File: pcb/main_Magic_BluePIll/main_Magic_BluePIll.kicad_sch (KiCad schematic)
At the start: 46 parts, among them J1 PW, J2 MPU6050, J3 ST_Link, J4 LiPo, J5 ESC, J9 Sensors, Q1 IRLML2502, SW1 Power_SW, SW4 BUTTON_Push, U1 BluePill_SWD_Breakout, U2 AMS1117CD-3.3, U6 CN3905

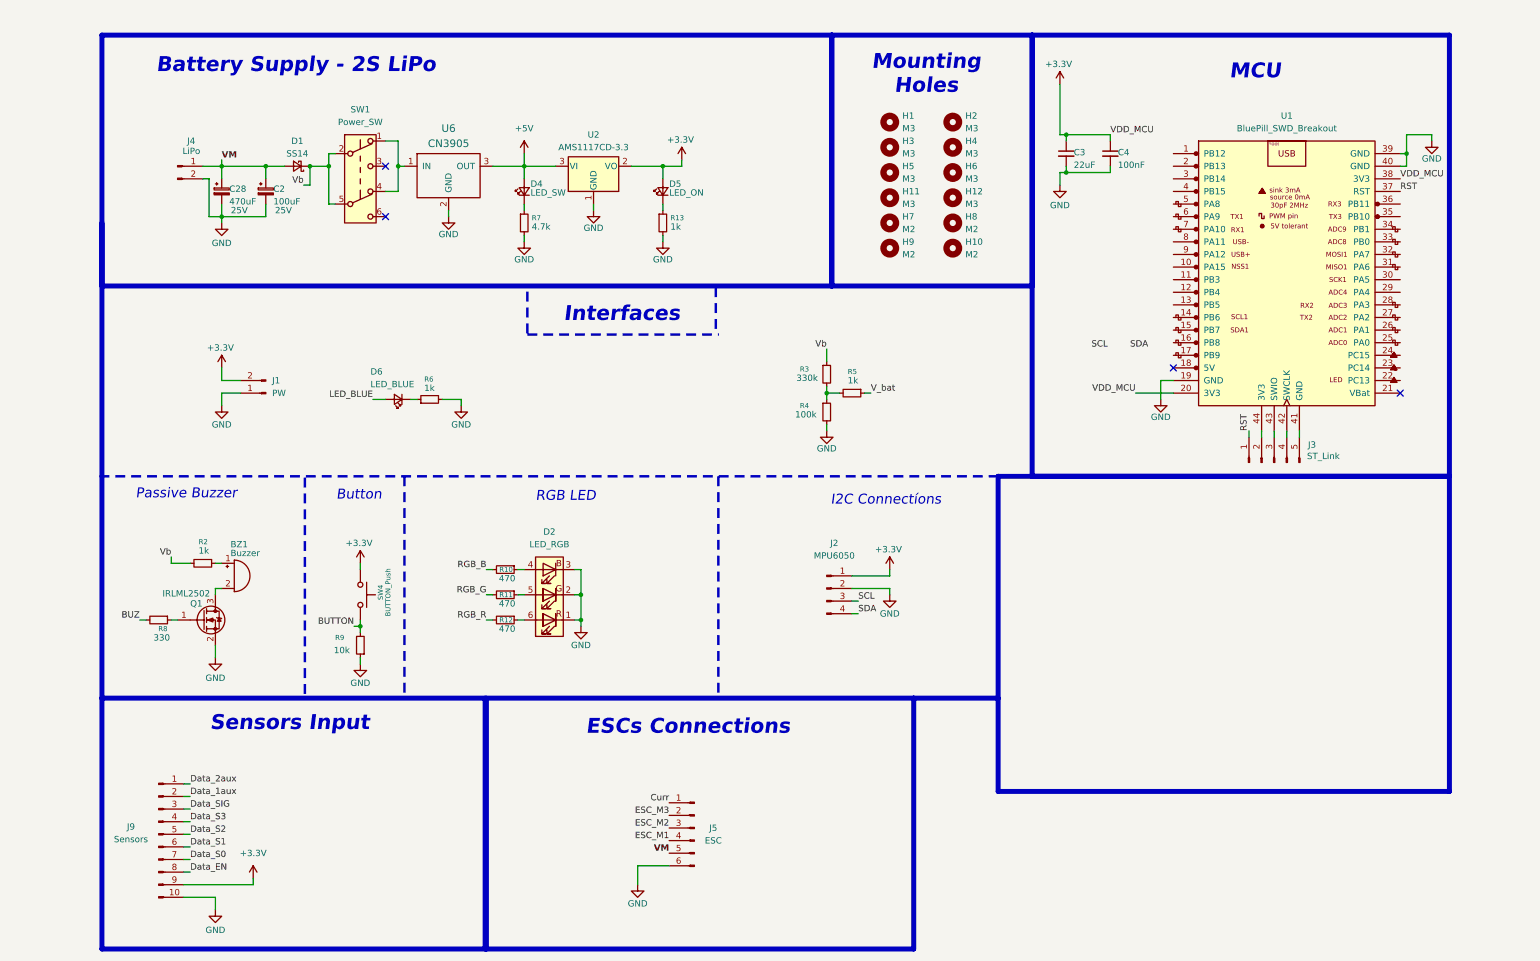
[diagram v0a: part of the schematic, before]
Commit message: bluepill pcb
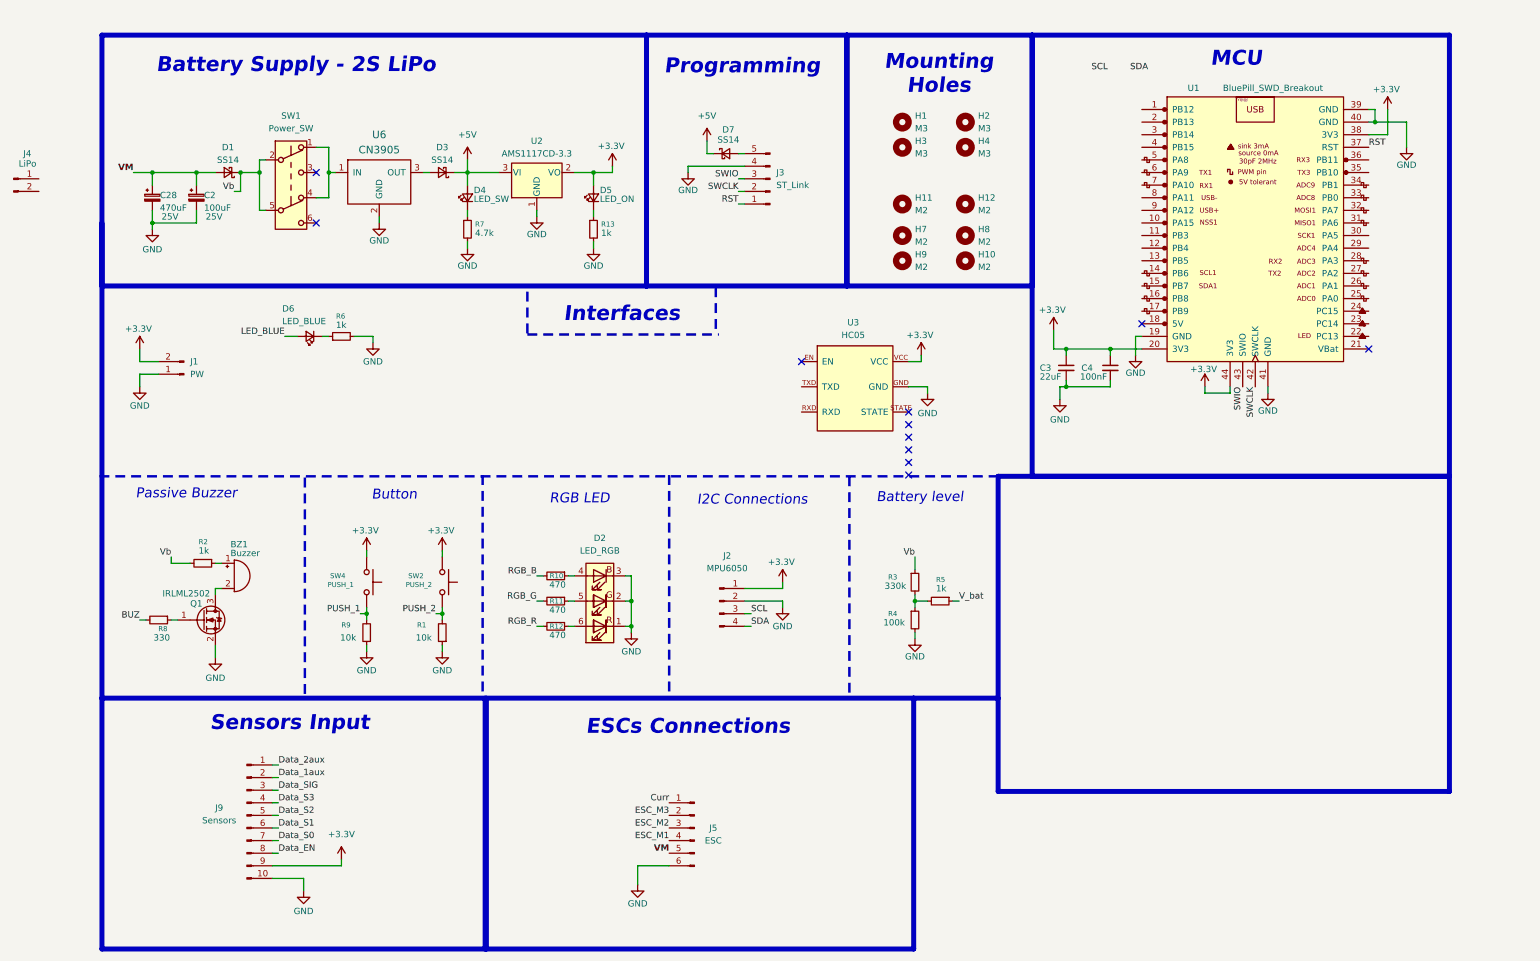
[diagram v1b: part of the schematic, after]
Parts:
- removed H5, H6: M3, MountingHole:MountingHole_3mm, symbol Mechanical:MountingHole
- added D3, D7: SS14, Diode_SMD:D_SMA, symbol Device:D_Schottky_Small
- added R1: 10k, Resistor_SMD:R_0805_2012Metric, symbol Device:R_Small
- added SW2: PUSH_2, MixLib:SW_Push_Sw-3424p_Handsolder, symbol Switch:SW_Push
- added U3: HC05, MixLib:HC05, symbol MixLib:HC05
- H11, H12: value M3 -> M2; footprint MountingHole:MountingHole_3mm -> MountingHole:MountingHole_2.2mm_M2
- J3: footprint Connector_PinHeader_2.54mm:PinHeader_1x05_P2.54mm_Horizontal -> Connector_PinHeader_2.54mm:PinHeader_1x05_P2.54mm_Vertical
- SW4: value BUTTON_Push -> PUSH_1
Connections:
- net +3.3V: now also U1.44 (3V3), SW2.1, U3.VCC
- net +5V: now also D3.1 (K), D7.1 (K); no longer U6.3 (OUT)
- net BUTTON: no longer R9.2, SW4.2
- net GND: now also J3.4 (Pin_4), U1.41 (GND), R1.1, U3.GND; no longer J4.2 (Pin_2)
- net VM: no longer J4.1 (Pin_1)
- net at J3.5 (Pin_5): now also D7.2 (A); no longer U1.41 (GND)
- net SWCLK: now reaches U1.42 (SWCLK)
- net SWCLK: now also J3.2 (Pin_2); no longer J3.4 (Pin_4)
- net SWIO: now reaches J3.3 (Pin_3), U1.43 (SWIO)
- new net: D3.2 (A), U6.3 (OUT)
- new net PUSH_1: R9.2, SW4.2
- new net PUSH_2: R1.2, SW2.2
- no-connect marks 4 -> 11
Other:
- note added: "Battery level"
- note added: "I2C Connections"
- note added: "Programming"
- note removed: "I2C Connectíons"
- moved on the sheet: C2, C28, C3, C4, D1, D2, D4, D5, D6, H1, H10, H2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
